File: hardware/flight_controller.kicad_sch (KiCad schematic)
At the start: 67 parts, among them IC1 BQ25883, IC2 STM32F722RET6, J1 Screw_Terminal_01x02, J3 USB-C, J4 MicroSD Socket, U1 BMP581, U2 TPS630702RNMR

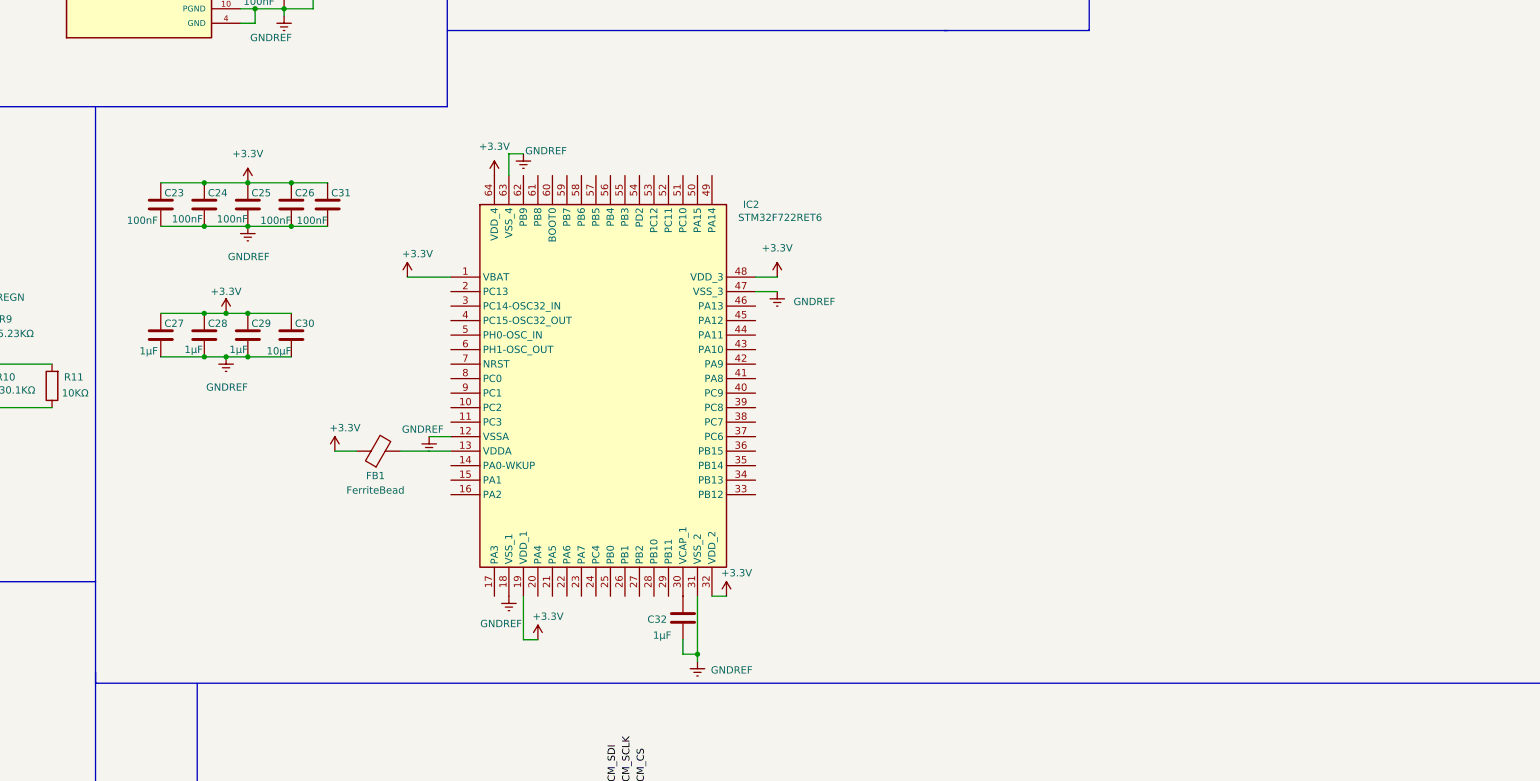
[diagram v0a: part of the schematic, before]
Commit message: stm32
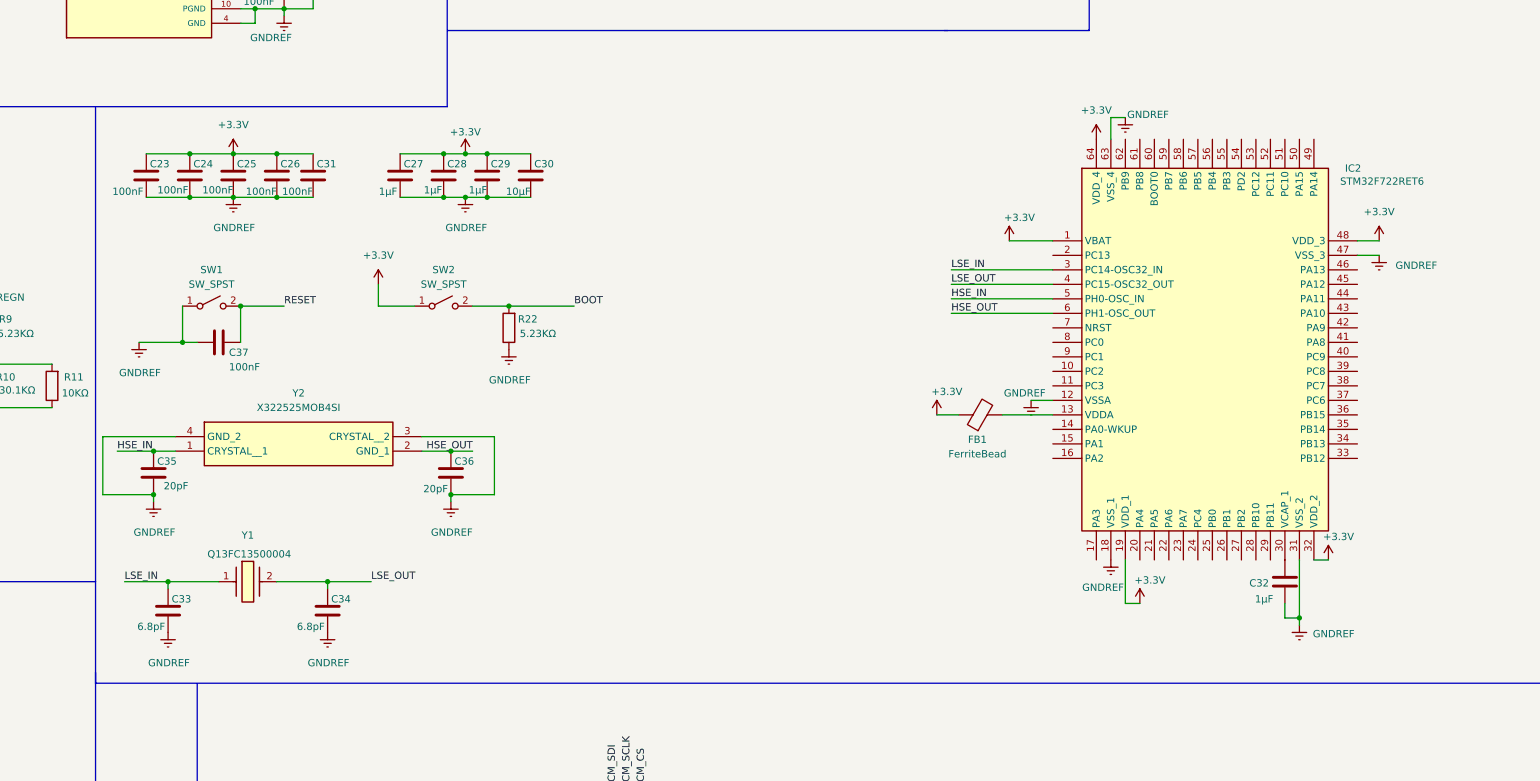
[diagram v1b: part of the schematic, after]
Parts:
- added C33, C34: 6.8pF, symbol Device:C
- added C35, C36: 20pF, symbol Device:C
- added C37: 100nF, symbol Device:C
- added R22: 5.23KΩ, symbol Device:R
- added SW1, SW2: SW_SPST, symbol Switch:SW_SPST
- added Y1: Q13FC13500004, drone_footprints:Q13FC13500004, symbol drone_symbols:Q13FC13500004
- added Y2: X322525MOB4SI, drone_footprints:X322525MOB4SI, symbol drone_symbols:X322525MOB4SI
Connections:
- net +3.3V: now also SW2.1 (A)
- net GND: now also C33.1, C34.1, C35.1, C36.1, C37.2, R22.1, SW1.1 (A), Y2.3 (CRYSTAL__2), Y2.4 (GND_2)
- net LSE_IN: now reaches IC2.3 (PC14-OSC32_IN)
- net LSE_IN: now also C33.2, Y1.1
- net LSE_OUT: now reaches IC2.4 (PC15-OSC32_OUT)
- net LSE_OUT: now also C34.2, Y1.2
- net HSE_IN: now reaches IC2.5 (PH0-OSC_IN)
- net HSE_IN: now also C35.2, Y2.1 (CRYSTAL__1)
- net HSE_OUT: now reaches IC2.6 (PH1-OSC_OUT)
- net HSE_OUT: now also C36.2, Y2.2 (GND_1)
- new net BOOT: R22.2, SW2.2 (B)
- new net RESET: C37.1, SW1.2 (B)
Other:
- moved on the sheet: C23, C24, C25, C26, C27, C28, C29, C30, C31, C32, FB1, IC2
